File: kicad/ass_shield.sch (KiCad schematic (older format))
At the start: 151 parts, among them J1 6-40V, J2 DEBUG, J3 5V, J4 UART2, J5 U.FL, J6 i2s, J7 SP, J8 U.FL, M1 CR1220SMD, Q1 BC817, U1 OPiZero, U2 DS3231M, U3 24LC256, U4 nRF24L01P, U5 PCF8574, U6 CC2530F, X1 USB_F1, X2 USB_F1, Y1 9,84375 MHz, Y2 13,5600 MHz, Y3 4,8970 MHz, Y4 6,7458 MHz, Y5 32 MHz, Y6 16 MHz, Y7 32 MHz

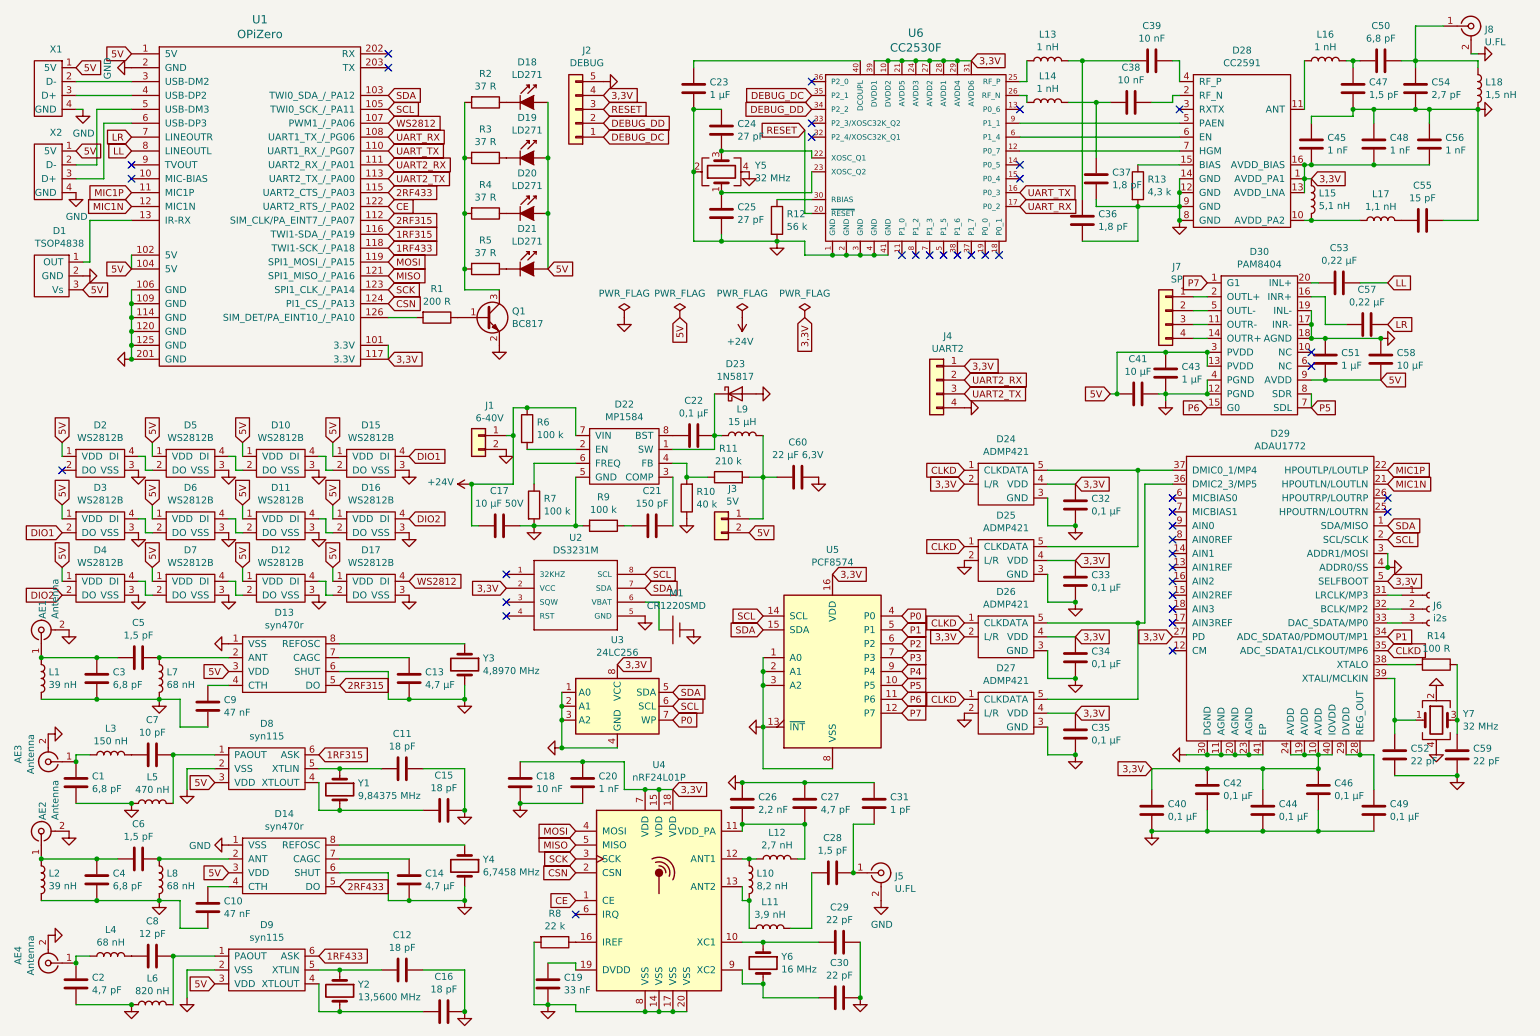
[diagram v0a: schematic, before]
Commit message: a msg
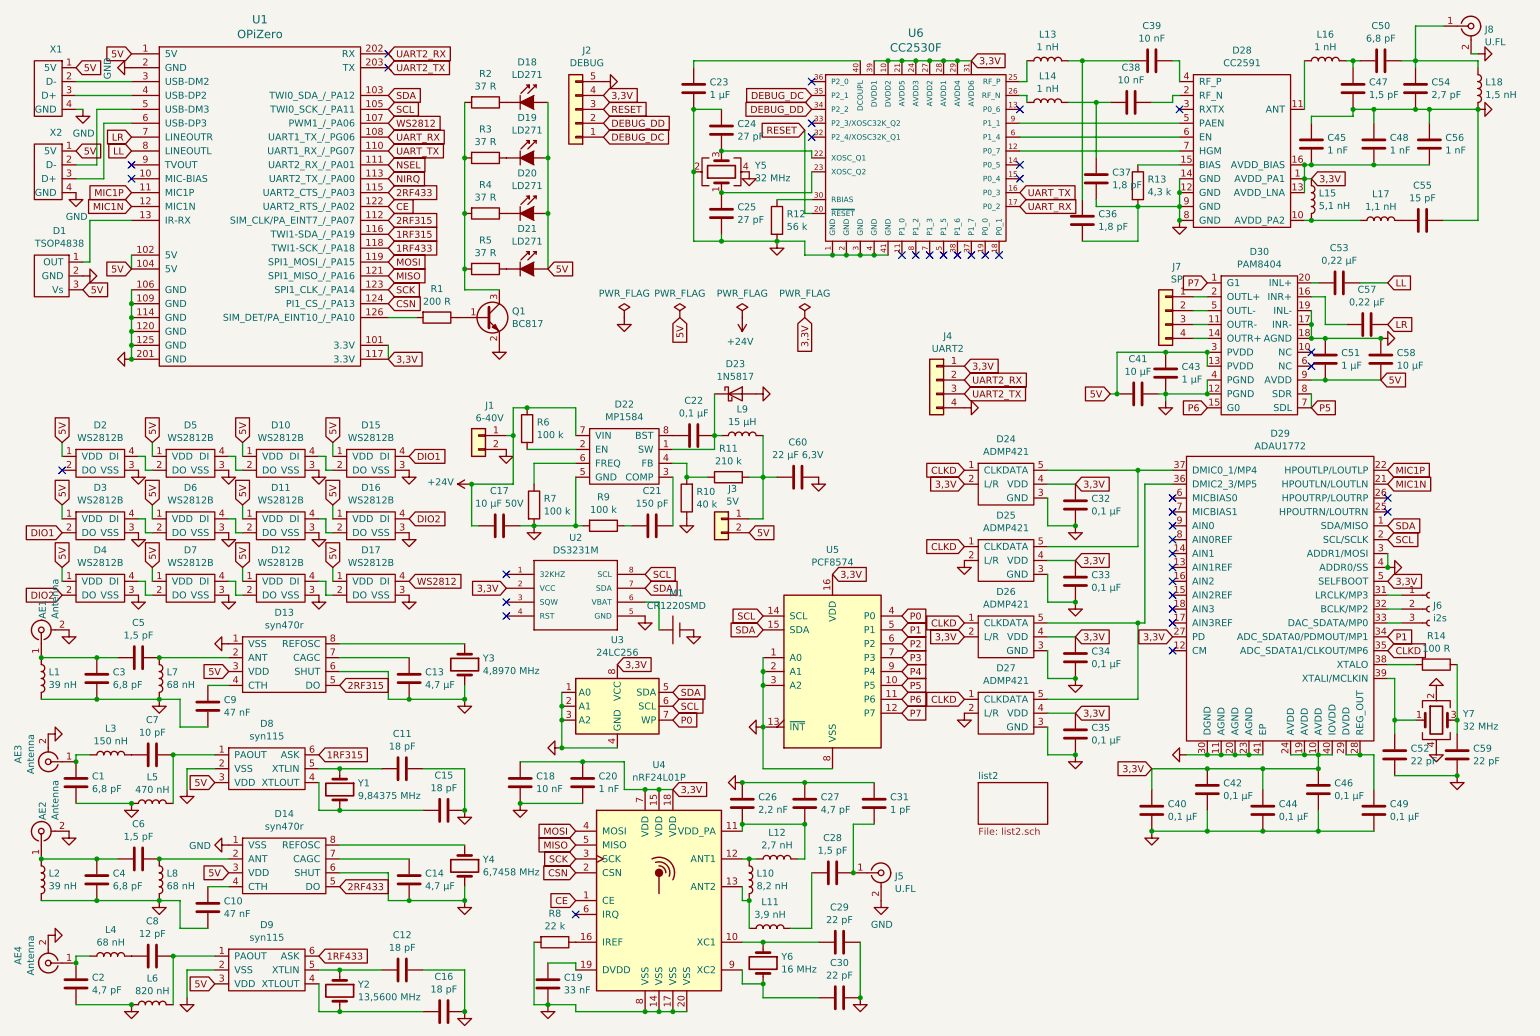
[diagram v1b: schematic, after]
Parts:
- Y6: footprint w_crystal:crystal_tc-38_horiz -> imm:Crystal_SMD_3215-2Pin_3.2x1.5mm
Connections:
- net UART2_RX: now also U1.202 (RX); no longer U1.111 (UART2_RX_/_PA01)
- net UART2_TX: now also U1.203 (TX); no longer U1.113 (UART2_TX_/_PA00)
- new net NIRQ: U1.113 (UART2_TX_/_PA00)
- new net NSEL: U1.111 (UART2_RX_/_PA01)
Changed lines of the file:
@@
 EESchema Schematic File Version 4
 LIBS:ass_shield-cache
-EELAYER 26 0
+EELAYER 29 0
 EELAYER END
 $Descr A4 11693 8268
 encoding utf-8
-Sheet 1 1
+Sheet 1 2
 Title ""
 Date ""
@@
 F 0 "Y6" V 5754 7481 50  0000 L CNN
 F 1 "16 MHz" V 5845 7481 50  0000 L CNN
-F 2 "w_crystal:crystal_tc-38_horiz" H 5800 7350 50  0001 C CNN
+F 2 "imm:Crystal_SMD_3215-2Pin_3.2x1.5mm" H 5800 7350 50  0001 C CNN
 F 3 "~" H 5800 7350 50  0001 C CNN
 	1    5800 7350
@@
 	0    -1   -1   0
 $EndComp
-Text GLabel 3100 1600 2    50   Input ~ 0
+Text GLabel 3100 800  2    50   Input ~ 0
 UART2_RX
-Text GLabel 3100 1700 2    50   Input ~ 0
+Text GLabel 3100 900  2    50   Input ~ 0
 UART2_TX
 Text GLabel 7250 3150 2    50   Input ~ 0
@@
 Connection ~ 600  5150
 $Comp
-L power:GND #PWR?
+L power:GND #PWR070
 U 1 1 5BE33315
 P 800 4950
-F 0 "#PWR?" H 800 4700 50  0001 C CNN
+F 0 "#PWR070" H 800 4700 50  0001 C CNN
 F 1 "GND" H 805 4777 50  0001 C CNN
 F 2 "" H 800 4950 50  0001 C CNN
@@
 Connection ~ 850  5900
 $Comp
-L power:GND #PWR?
+L power:GND #PWR063
 U 1 1 5BE9F8EF
 P 650 5700
-F 0 "#PWR?" H 650 5450 50  0001 C CNN
+F 0 "#PWR063" H 650 5450 50  0001 C CNN
 F 1 "GND" H 655 5527 50  0001 C CNN
 F 2 "" H 650 5700 50  0001 C CNN
@@
 Connection ~ 600  6600
 $Comp
-L power:GND #PWR?
+L power:GND #PWR071
 U 1 1 5BF0C4AF
 P 800 6400
-F 0 "#PWR?" H 800 6150 50  0001 C CNN
+F 0 "#PWR071" H 800 6150 50  0001 C CNN
 F 1 "GND" H 805 6227 50  0001 C CNN
 F 2 "" H 800 6400 50  0001 C CNN
@@
 Connection ~ 850  7350
 $Comp
-L power:GND #PWR?
+L power:GND #PWR069
 U 1 1 5BF79106
 P 650 7150
-F 0 "#PWR?" H 650 6900 50  0001 C CNN
+F 0 "#PWR069" H 650 6900 50  0001 C CNN
 F 1 "GND" H 655 6977 50  0001 C CNN
 F 2 "" H 650 7150 50  0001 C CNN
@@
 	0    -1   -1   0
 $EndComp
+$Sheet
+S 7350 6050 500  300
+U 5BE401CA
+F0 "list2" 50
+F1 "list2.sch" 50
+$EndSheet
+Text GLabel 3100 1600 2    50   Input ~ 0
+NSEL
+Text GLabel 3100 1700 2    50   Input ~ 0
+NIRQ
 $EndSCHEMATC
